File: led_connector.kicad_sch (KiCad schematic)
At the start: 7 parts, among them U3 SM02B-SRSS-TB-LF-SN, U4 SM02B-SRSS-TB-LF-SN

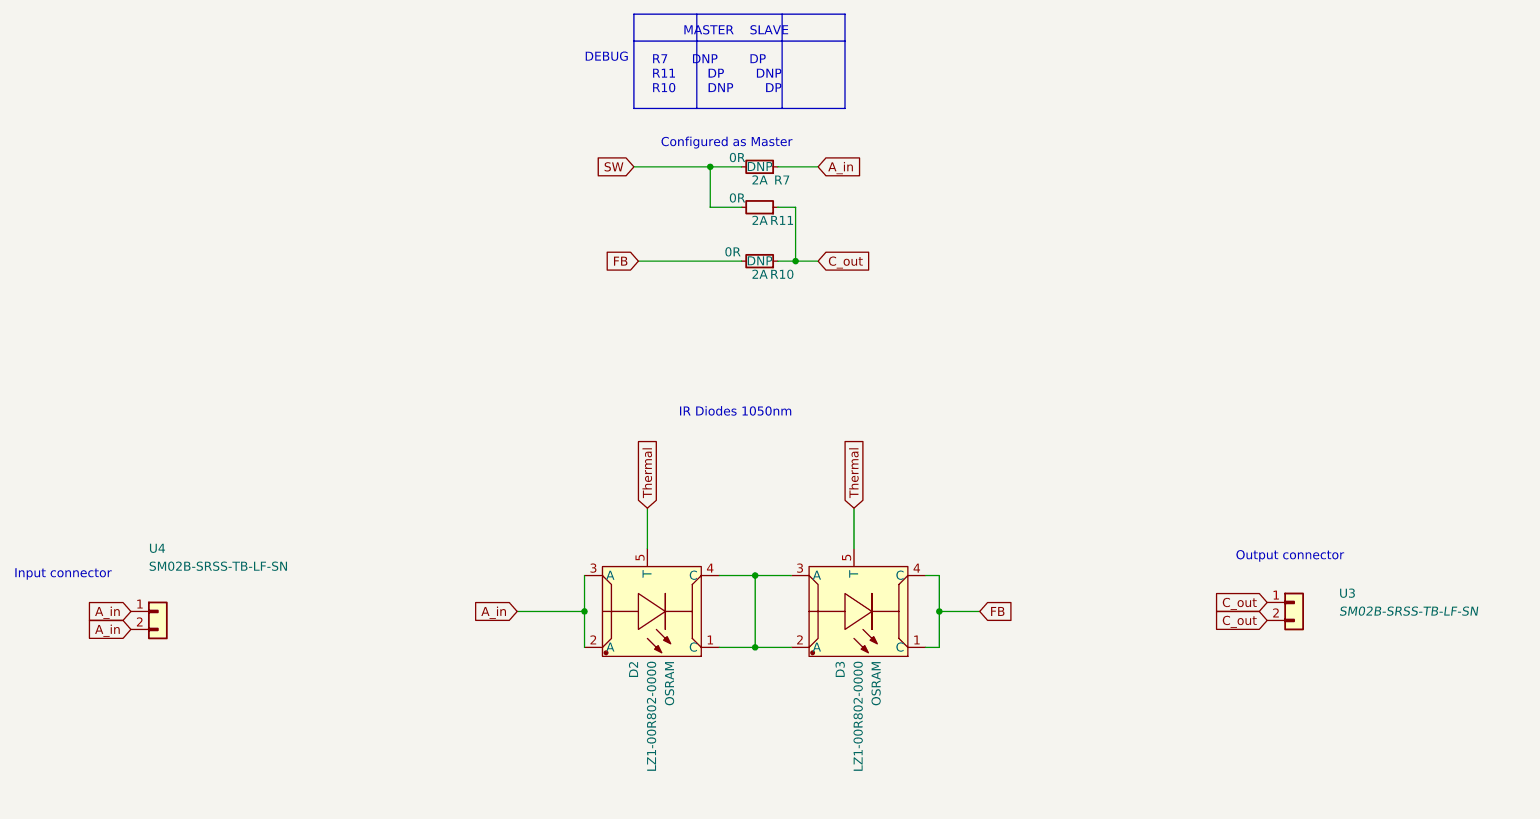
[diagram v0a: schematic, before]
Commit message: Refresh standardization on schematic and PCB
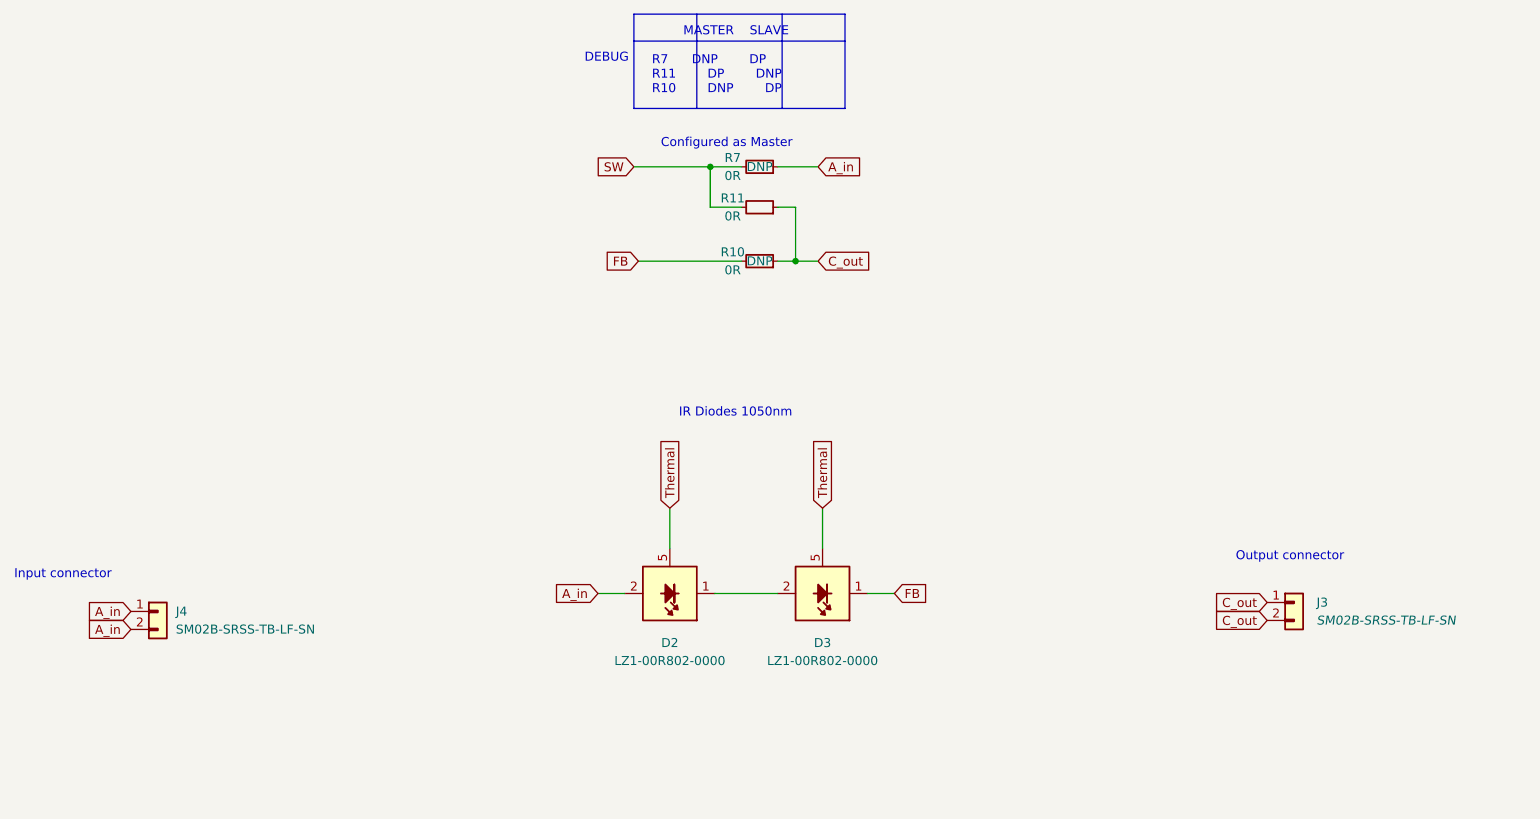
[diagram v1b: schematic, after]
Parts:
- D2, D3: footprint antmicro-footprints:LZ1-00R802_4EP_4.4x4.4 -> antmicro-footprints:LED_IR_LZ1-00R802; symbol antmicroLEDIndicationDiscrete:LZ1-00R802-0000 -> antmicroLEDIndicationDiscrete:LED_IR_LZ1-00R802; Author (none) -> Antmicro; License Apache-2.0 License -> Apache-2.0; Manufacturer OSRAM -> Osram
- R10, R11, R7: Author (none) -> Antmicro; Copyright Copyright (c) 2023 Antmicro -> (none); License Apache-2.0 License -> Apache-2.0; Manufacturer Multicomp PRO -> Multicomp
- renumbered U3 to J3, U4 to J4
